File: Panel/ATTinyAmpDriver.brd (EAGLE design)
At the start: 50 x 50 mm, 44 parts, among them Q1 SI2301CDS, Q2 BC846, U1 SPX5205M5-L-3-3, U2 ATTINY5-TSHR, U3 MCP6L2-X_SN

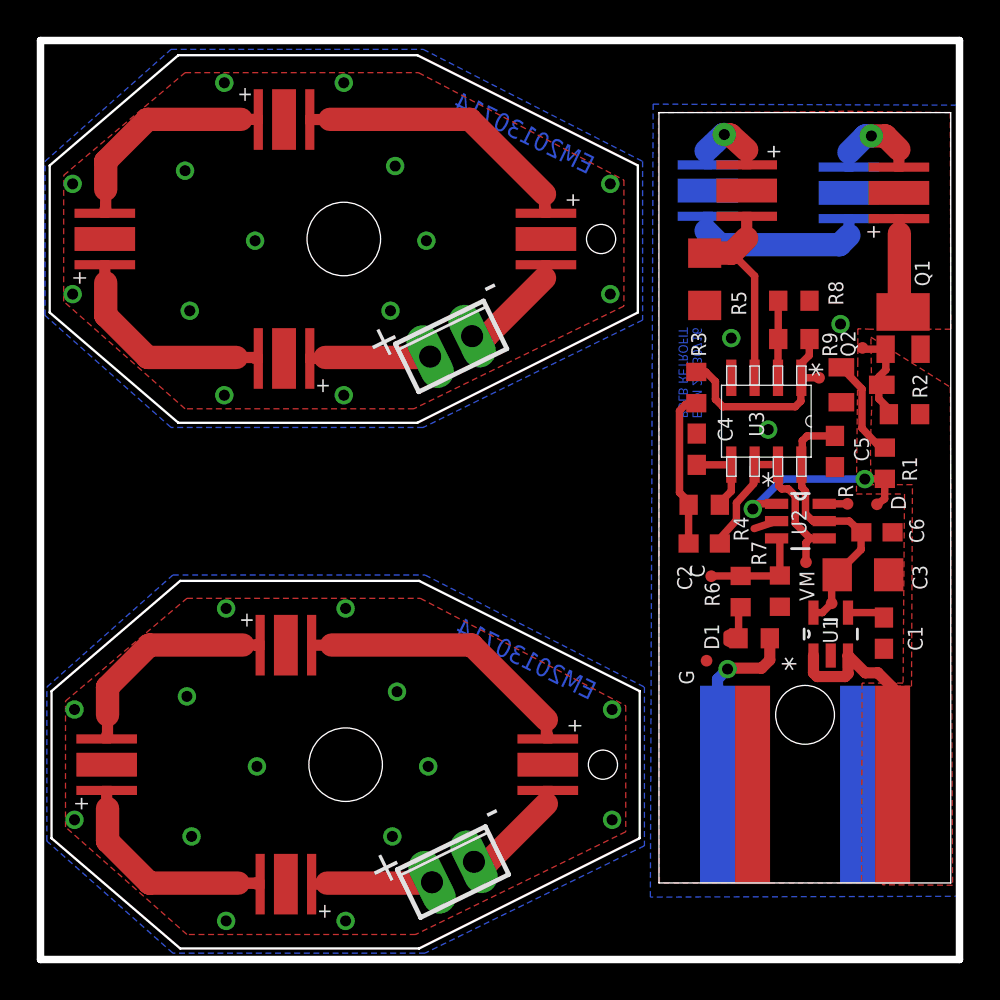
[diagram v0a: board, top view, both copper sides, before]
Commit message: Turn and Tail combined Panel
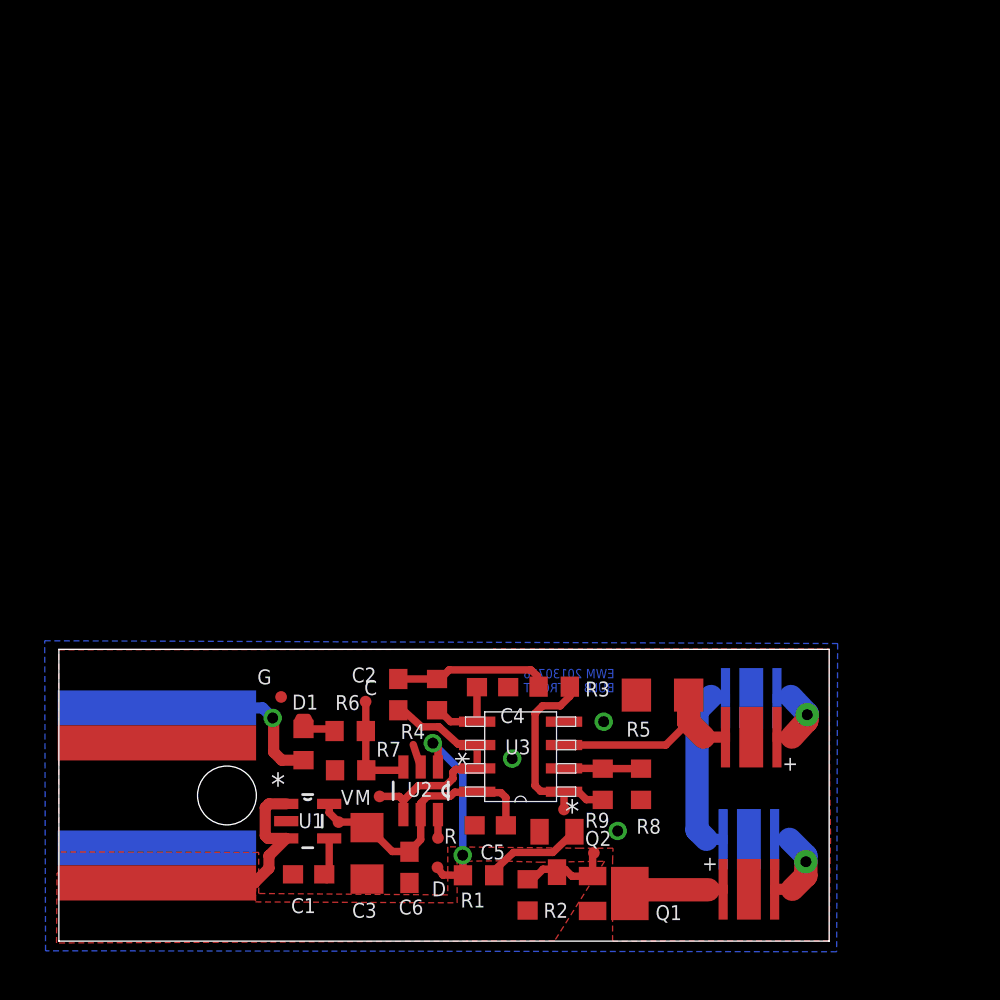
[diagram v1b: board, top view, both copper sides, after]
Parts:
- removed LED10, LED11, LED12, LED5, LED6, LED7, LED8, LED9: LUXEON_REBELCREE_XP-E, Combined:CREE_XP-E
- removed X1, X2: (no value), con-phoenix-254:2POL254
- moved U$1 35.3 mm to (5.33, 7.92), turned to 90 degrees
- moved LED3 35.3 mm to (37.7, 13.2), flipped to the bottom, turned to 180 degrees
- moved Q1 35.0 mm to (31.1, 2.59), turned to 270 degrees
- moved C1 33.9 mm to (13.6, 3.63), turned to 180 degrees
- moved R2 33.2 mm to (25.5, 2.51), turned to 90 degrees
- moved R1 31.5 mm to (22.8, 3.58), turned to 0 degrees
- moved C6 31.3 mm to (19.1, 4.01), turned to 270 degrees
- moved PWM 31.1 mm to (29.1, 4.80), turned to 0 degrees
- moved TPIDATA 31.0 mm to (20.6, 4.01), turned to 0 degrees
- moved C3 30.9 mm to (16.8, 4.78), turned to 270 degrees
- moved Q2 30.3 mm to (27.1, 4.85), turned to 180 degrees
- moved U1 30.2 mm to (13.5, 6.53), turned to 0 degrees
- moved +5V 29.4 mm to (15.2, 6.48), turned to 0 degrees
- moved RESET 28.8 mm to (20.6, 5.61), turned to 0 degrees
- moved C5 27.7 mm to (23.5, 6.30), turned to 180 degrees
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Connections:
- removed net N$1 (its old number): LED5.AN, LED6.CT
- removed net N$13: LED11.CT, LED12.AN
- removed net N$14: LED9.AN, Q1.P$3
- removed net N$15: LED10.AN, LED9.CT
- removed net N$2 (its old number): LED1.AN, LED2.CT
- removed net N$4 (its old number): LED3.AN, LED4.CT
- removed net N$5 (its old number): LED6.AN, LED7.CT
- removed net N$6 (its old number): LED7.AN, LED8.CT
- removed net THERMAL: LED1.TH, LED2.TH, LED3.TH, LED4.TH
- removed net THERMAL1: LED5.TH, LED6.TH, LED7.TH, LED8.TH
- removed net V+: LED4.AN, X1.1
- removed net V+1: LED8.AN, X2.1
- removed net V-: LED1.CT, X1.2
- removed net V-1: LED5.CT, X2.2
- new net N$10: LED3.CT, LED4.AN
- new net N$7: LED1.CT, LED2.AN
- net CROSSOVER: now also LED2.CT, LED3.AN; no longer LED10.CT, LED11.AN
- net D-: now also LED4.CT; no longer LED12.CT
- net GND: now also LED1.TH, LED2.TH, LED3.TH, LED4.TH; no longer LED10.TH, LED11.TH, LED12.TH, LED9.TH
- net N$3: now also LED1.AN, Q1.P$3; no longer LED2.AN, LED3.CT
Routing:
- net N$1 (its old number): track 15.1 -> 0.00 mm
- net N$2 (its old number): track 15.1 -> 0.00 mm
- net N$5 (its old number): track 11.7 -> 0.00 mm
- net N$6 (its old number): track 11.6 -> 0.00 mm
- net N$4 (its old number): track 11.6 -> 0.00 mm
- net N$3: track 11.7 -> 4.97 mm
- net V+1: track 6.39 -> 0.00 mm
- net V+: track 6.39 -> 0.00 mm
- net V-: track 5.81 -> 0.00 mm
- net V-1: track 5.81 -> 0.00 mm
- net N$14: track 4.97 -> 0.00 mm
- net N$7: track 0.00 -> 4.76 mm, vias 0 -> 1
- net N$15: track 4.76 -> 0.00 mm, vias 1 -> 0
- net N$10: track 0.00 -> 4.06 mm, vias 0 -> 1
- net N$13: track 4.06 -> 0.00 mm, vias 1 -> 0
- removed copper zone on layer 1, net THERMAL
- removed copper zone on layer 16, net THERMAL
- removed copper zone on layer 1, net THERMAL1
- removed copper zone on layer 16, net THERMAL1
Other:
- board size 50 x 50 mm -> 41.9 x 15.9 mm
- board text removed: "+"
- board text removed: "-"
- board text removed: "EM20130714"
